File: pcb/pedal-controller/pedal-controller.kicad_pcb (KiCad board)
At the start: 2 copper layers, 4 parts

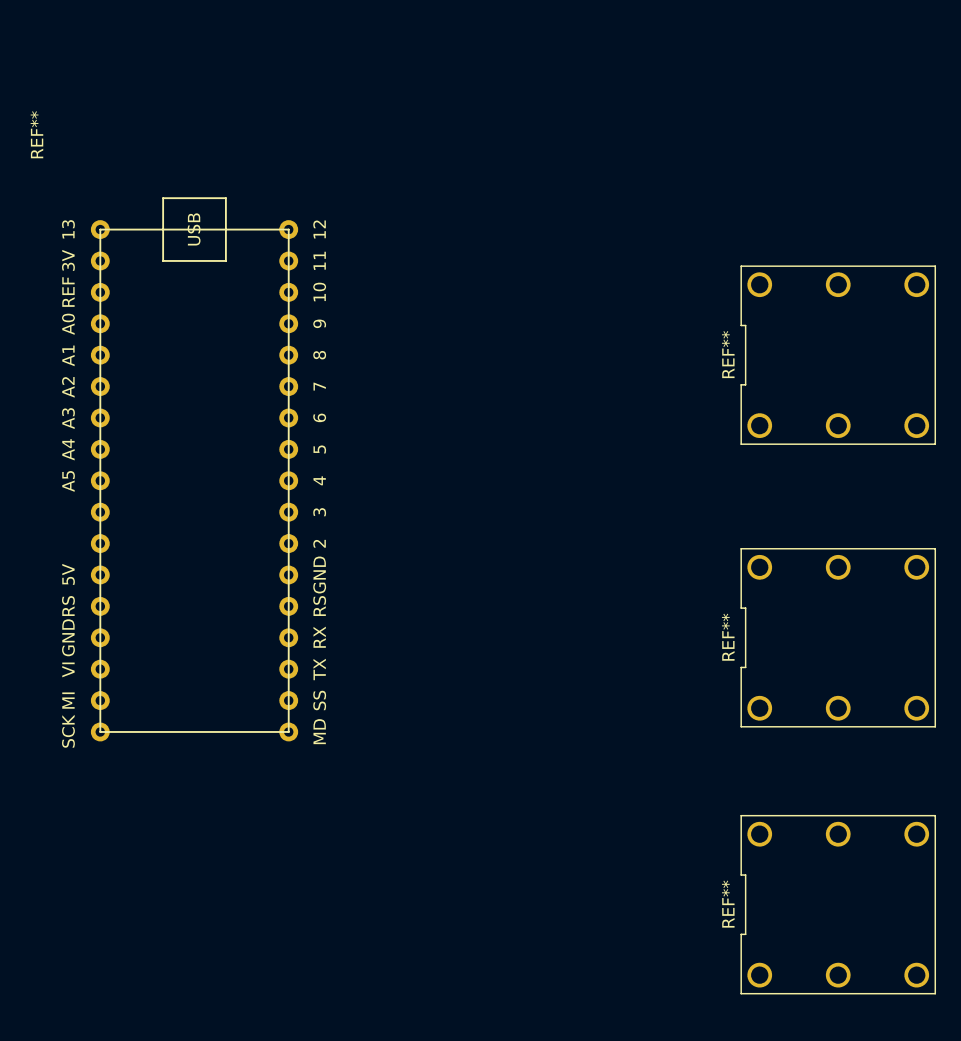
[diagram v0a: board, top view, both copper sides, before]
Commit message: ordered version
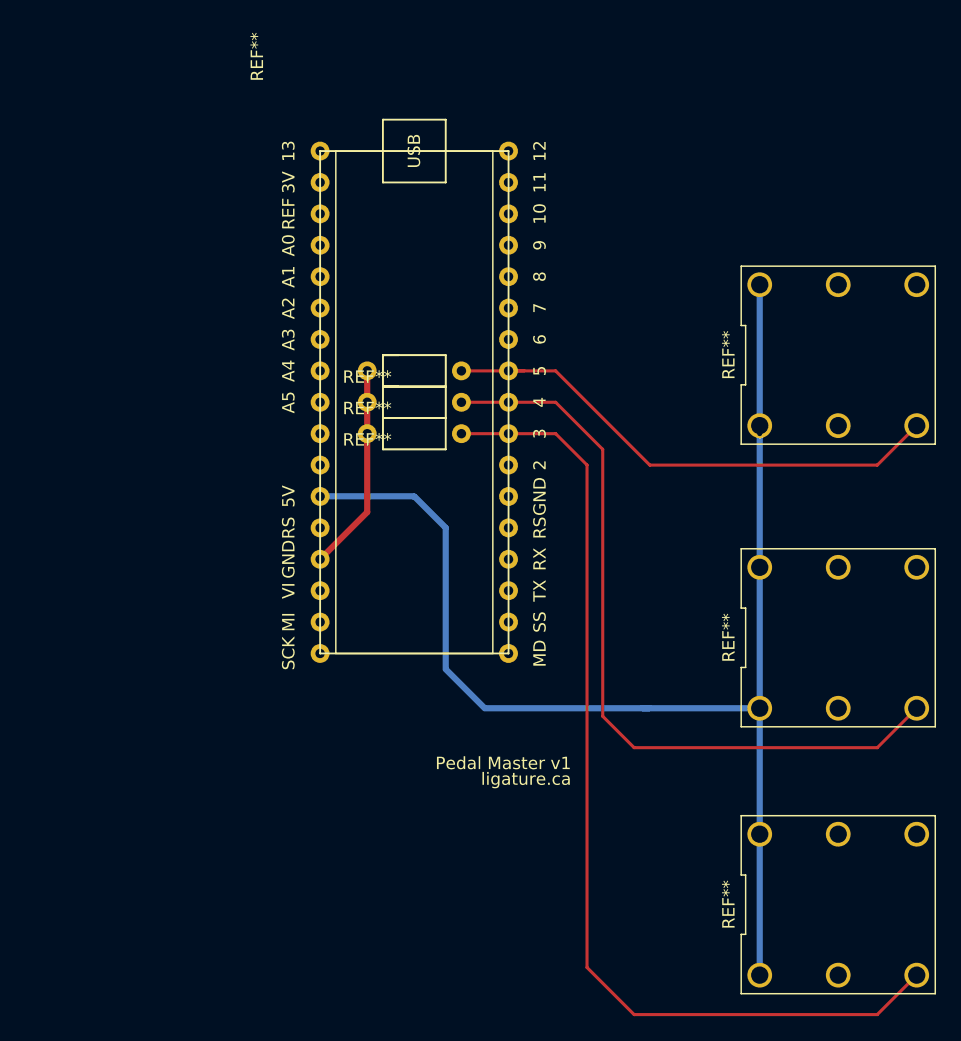
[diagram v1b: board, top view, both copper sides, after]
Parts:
- added REF**: 10K, pedal-controller:resistor, F.Cu at (237.5, 35.6)
- added REF**: 10K, pedal-controller:resistor, F.Cu at (237.5, 40.6)
- added REF**: 10K, pedal-controller:resistor, F.Cu at (237.5, 38.1)
- moved REF** 18.9 mm to (233.7, 17.8)
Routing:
- net (no net): track 0.00 -> 309.7 mm, vias 0 -> 1
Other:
- board text added: "Pedal Master v1"
- board text added: "ligature.ca"
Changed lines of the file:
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@@
   (general
     (thickness 1.6)
-    (drawings 0)
-    (tracks 0)
+    (drawings 17)
+    (tracks 34)
     (zones 0)
-    (modules 4)
+    (modules 7)
     (nets 1)
   )
@@
     (solder_mask_min_width 0.25)
     (aux_axis_origin 0 0)
-    (visible_elements FFFFFF7F)
+    (visible_elements FFFFF77F)
     (pcbplotparams
       (layerselection 0x010fc_ffffffff)
@@
       (outputformat 1)
       (mirror false)
-      (drillshape 1)
+      (drillshape 0)
       (scaleselection 1)
-      (outputdirectory ""))
+      (outputdirectory "export/"))
   )
   (net 0 "")
@@
     (uvia_drill 0.1)
   )
+  (module pedal-controller:resistor (layer F.Cu)
+    (at 237.49 35.56)
+    (fp_text reference REF** (at 0 0.5) (layer F.SilkS)
+      (effects (font (size 1 1) (thickness 0.15)))
+    )
+    (fp_text value 10K (at 3.81 0) (layer F.Fab)
+      (effects (font (size 1 1) (thickness 0.15)))
+    )
+    (fp_line (start 1.27 -1.27) (end 2.54 -1.27) (layer F.SilkS) (width 0.15))
+    (fp_line (start 6.35 -1.27) (end 1.27 -1.27) (layer F.SilkS) (width 0.15))
+    (fp_line (start 6.35 1.27) (end 6.35 -1.27) (layer F.SilkS) (width 0.15))
+    (fp_line (start 1.27 1.27) (end 6.35 1.27) (layer F.SilkS) (width 0.15))
+    (fp_line (start 1.27 -1.27) (end 1.27 1.27) (layer F.SilkS) (width 0.15))
+    (pad 2 thru_hole circle (at 7.62 0) (size 1.524 1.524) (drill 0.762) (layers *.Cu *.Mask))
+    (pad 1 thru_hole circle (at 0 0) (size 1.524 1.524) (drill 0.762) (layers *.Cu *.Mask))
+  )
+  (module pedal-controller:resistor (layer F.Cu)
+    (at 237.49 40.64)
+    (fp_text reference REF** (at 0 0.5) (layer F.SilkS)
+      (effects (font (size 1 1) (thickness 0.15)))
+    )
+    (fp_text value 10K (at 3.81 0) (layer F.Fab)
+      (effects (font (size 1 1) (thickness 0.15)))
+    )
+    (fp_line (start 1.27 -1.27) (end 2.54 -1.27) (layer F.SilkS) (width 0.15))
+    (fp_line (start 6.35 -1.27) (end 1.27 -1.27) (layer F.SilkS) (width 0.15))
+    (fp_line (start 6.35 1.27) (end 6.35 -1.27) (layer F.SilkS) (width 0.15))
+    (fp_line (start 1.27 1.27) (end 6.35 1.27) (layer F.SilkS) (width 0.15))
+    (fp_line (start 1.27 -1.27) (end 1.27 1.27) (layer F.SilkS) (width 0.15))
+    (pad 2 thru_hole circle (at 7.62 0) (size 1.524 1.524) (drill 0.762) (layers *.Cu *.Mask))
+    (pad 1 thru_hole circle (at 0 0) (size 1.524 1.524) (drill 0.762) (layers *.Cu *.Mask))
+  )
+  (module pedal-controller:resistor (layer F.Cu)
+    (at 237.49 38.1)
+    (fp_text reference REF** (at 0 0.5) (layer F.SilkS)
+      (effects (font (size 1 1) (thickness 0.15)))
+    )
+    (fp_text value 10K (at 3.81 0) (layer F.Fab)
+      (effects (font (size 1 1) (thickness 0.15)))
+    )
+    (fp_line (start 1.27 -1.27) (end 2.54 -1.27) (layer F.SilkS) (width 0.15))
+    (fp_line (start 6.35 -1.27) (end 1.27 -1.27) (layer F.SilkS) (width 0.15))
+    (fp_line (start 6.35 1.27) (end 6.35 -1.27) (layer F.SilkS) (width 0.15))
+    (fp_line (start 1.27 1.27) (end 6.35 1.27) (layer F.SilkS) (width 0.15))
+    (fp_line (start 1.27 -1.27) (end 1.27 1.27) (layer F.SilkS) (width 0.15))
+    (pad 2 thru_hole circle (at 7.62 0) (size 1.524 1.524) (drill 0.762) (layers *.Cu *.Mask))
+    (pad 1 thru_hole circle (at 0 0) (size 1.524 1.524) (drill 0.762) (layers *.Cu *.Mask))
+  )
   (module pedal-controller:Arduino_Micro (layer F.Cu)
-    (at 215.9 24.13 270)
+    (at 233.68 17.78 270)
     (fp_text reference REF** (at -7.62 5.08 90) (layer F.SilkS)
       (effects (font (size 1 1) (thickness 0.15)))
@@
     (pad 6 thru_hole circle (at -6.35 -5.7) (size 2 2) (drill 1.4) (layers *.Cu *.Mask))
   )
+  (gr_text "Pedal Master v1" (at 254 67.31) (layer F.SilkS)
+    (effects (font (size 1 1) (thickness 0.15)) (justify right))
+  )
+  (gr_text ligature.ca (at 254 68.58) (layer F.SilkS)
+    (effects (font (size 1 1) (thickness 0.15)) (justify right))
+  )
+  (gr_line (start 247.65 17.78) (end 234.95 17.78) (layer F.SilkS) (width 0.12))
+  (gr_line (start 247.65 58.42) (end 247.65 17.78) (layer F.SilkS) (width 0.12))
+  (gr_line (start 234.95 58.42) (end 247.65 58.42) (layer F.SilkS) (width 0.12))
+  (gr_line (start 234.95 17.78) (end 234.95 58.42) (layer F.SilkS) (width 0.12))
+  (gr_line (start 238.76 41.91) (end 238.76 39.37) (layer F.SilkS) (width 0.12))
+  (gr_line (start 243.84 41.91) (end 238.76 41.91) (layer F.SilkS) (width 0.12))
+  (gr_line (start 238.76 39.37) (end 243.84 39.37) (layer F.SilkS) (width 0.12))
+  (gr_line (start 238.76 39.37) (end 238.76 36.83) (layer F.SilkS) (width 0.12))
+  (gr_line (start 243.84 39.37) (end 238.76 39.37) (layer F.SilkS) (width 0.12))
+  (gr_line (start 243.84 36.83) (end 243.84 39.37) (layer F.SilkS) (width 0.12))
+  (gr_line (start 238.76 36.83) (end 243.84 36.83) (layer F.SilkS) (width 0.12))
+  (gr_line (start 238.76 36.83) (end 238.76 34.29) (layer F.SilkS) (width 0.12))
+  (gr_line (start 243.84 36.83) (end 238.76 36.83) (layer F.SilkS) (width 0.12))
+  (gr_line (start 243.84 34.29) (end 243.84 36.83) (layer F.SilkS) (width 0.12))
+  (gr_line (start 238.76 34.29) (end 243.84 34.29) (layer F.SilkS) (width 0.12))
+  (segment (start 269.24 62.85) (end 269.24 73.04) (width 0.5) (layer B.Cu) (net 0) (status 30))
+  (segment (start 248.92 35.56) (end 245.11 35.56) (width 0.25) (layer F.Cu) (net 0) (status 30))
+  (segment (start 248.92 38.1) (end 245.11 38.1) (width 0.25) (layer F.Cu) (net 0) (status 30))
+  (segment (start 248.92 40.64) (end 245.11 40.64) (width 0.25) (layer F.Cu) (net 0) (status 30))
+  (segment (start 269.24 40.64) (end 269.24 39.99) (width 0.25) (layer B.Cu) (net 0) (status 30))
+  (segment (start 269.24 73.04) (end 269.24 84.44) (width 0.5) (layer B.Cu) (net 0) (status 30))
+  (segment (start 269.24 62.85) (end 269.24 28.59) (width 0.5) (layer B.Cu) (net 0) (status 30))
+  (segment (start 241.3 45.72) (end 243.84 48.26) (width 0.5) (layer B.Cu) (net 0))
+  (segment (start 233.68 45.72) (end 241.3 45.72) (width 0.5) (layer B.Cu) (net 0) (status 10))
+  (segment (start 243.84 48.26) (end 243.84 59.69) (width 0.5) (layer B.Cu) (net 0))
+  (segment (start 243.84 59.69) (end 247 62.85) (width 0.5) (layer B.Cu) (net 0))
+  (segment (start 247 62.85) (end 260.35 62.85) (width 0.5) (layer B.Cu) (net 0))
+  (segment (start 259.08 87.63) (end 278.75 87.63) (width 0.25) (layer F.Cu) (net 0))
+  (segment (start 278.75 87.63) (end 281.94 84.44) (width 0.25) (layer F.Cu) (net 0) (status 20))
+  (segment (start 255.27 83.82) (end 259.08 87.63) (width 0.25) (layer F.Cu) (net 0))
+  (segment (start 252.73 40.64) (end 255.27 43.18) (width 0.25) (layer F.Cu) (net 0))
+  (segment (start 248.92 40.64) (end 252.73 40.64) (width 0.25) (layer F.Cu) (net 0) (status 10))
+  (segment (start 255.27 43.18) (end 255.27 83.82) (width 0.25) (layer F.Cu) (net 0))
+  (segment (start 237.49 35.56) (end 237.49 46.99) (width 0.5) (layer F.Cu) (net 0) (status 10))
+  (segment (start 237.49 46.99) (end 233.68 50.8) (width 0.5) (layer F.Cu) (net 0) (status 20))
+  (segment (start 260.35 43.18) (end 278.75 43.18) (width 0.25) (layer F.Cu) (net 0))
+  (segment (start 278.75 43.18) (end 281.94 39.99) (width 0.25) (layer F.Cu) (net 0) (status 20))
+  (segment (start 252.73 35.56) (end 260.35 43.18) (width 0.25) (layer F.Cu) (net 0))
+  (segment (start 248.92 35.56) (end 252.73 35.56) (width 0.25) (layer F.Cu) (net 0) (status 10))
+  (segment (start 259.08 66.04) (end 278.75 66.04) (width 0.25) (layer F.Cu) (net 0))
+  (segment (start 278.75 66.04) (end 281.94 62.85) (width 0.25) (layer F.Cu) (net 0) (status 20))
+  (segment (start 256.54 63.5) (end 259.08 66.04) (width 0.25) (layer F.Cu) (net 0))
+  (segment (start 256.54 41.91) (end 256.54 63.5) (width 0.25) (layer F.Cu) (net 0))
+  (segment (start 252.73 38.1) (end 256.54 41.91) (width 0.25) (layer F.Cu) (net 0))
+  (segment (start 248.92 38.1) (end 252.73 38.1) (width 0.25) (layer F.Cu) (net 0) (status 10))
+  (segment (start 259.73 62.85) (end 269.24 62.85) (width 0.5) (layer B.Cu) (net 0) (status 20))
+  (segment (start 250.19 35.56) (end 248.92 35.56) (width 0.25) (layer F.Cu) (net 0) (status 20))
+  (segment (start 248.92 40.64) (end 248.92 40.64) (width 0.25) (layer F.Cu) (net 0))
+  (via (at 269.24 40.64) (size 0.8) (drill 0.4) (layers F.Cu B.Cu) (net 0))
 )
